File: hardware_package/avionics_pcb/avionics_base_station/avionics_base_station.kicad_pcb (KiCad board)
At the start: 2 copper layers, 33 x 52.7 mm, 9 parts, among them J1 ANT, J2 GND_PASS, U1 NODEMCU, U2 RFM98

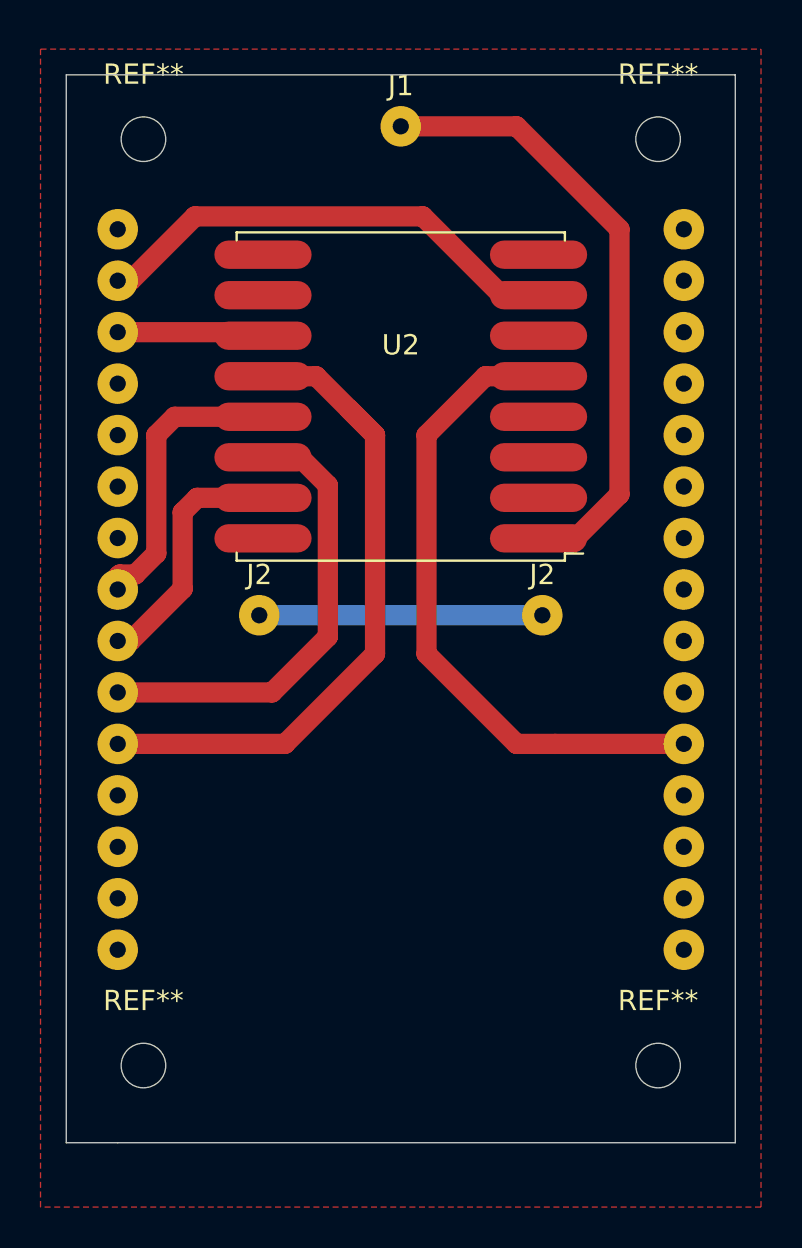
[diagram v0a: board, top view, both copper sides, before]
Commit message: updated the base station PCB
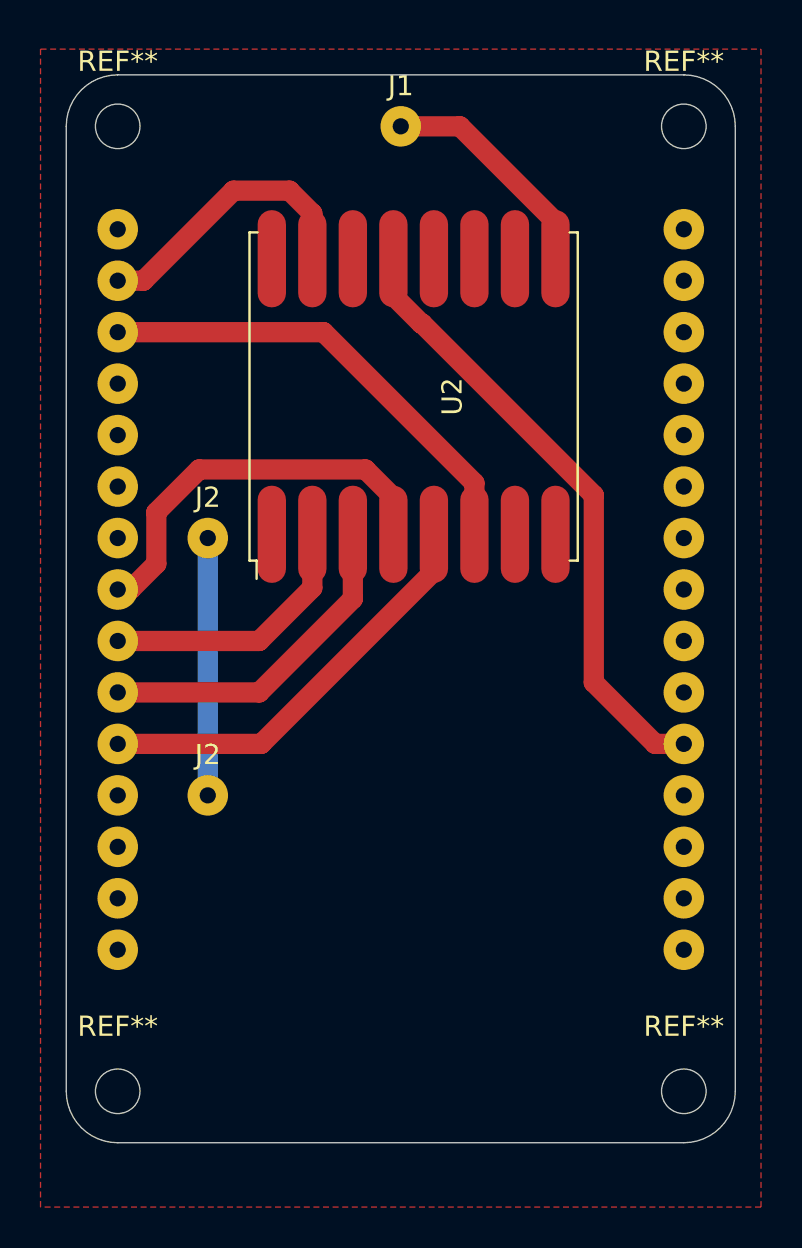
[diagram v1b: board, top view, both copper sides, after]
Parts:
- removed the REF** at (67.3, 38.7)
- removed the REF** at (41.9, 38.7)
- removed the REF** at (67.3, 84.5)
- added REF**: MountingHole_2.2mm_M2, MountingHole:MountingHole_2.2mm_M2, F.Cu at (68.6, 38.1)
- added REF**: MountingHole_2.2mm_M2, MountingHole:MountingHole_2.2mm_M2, F.Cu at (40.6, 38.1)
- added REF**: M2, MountingHole:MountingHole_2.2mm_M2, F.Cu at (68.6, 85.7)
- moved J2 18.8 mm to (45.1, 71.1)
- moved J2 4.58 mm to (45.1, 58.4)
- moved REF** 1.80 mm to (40.6, 85.7)
- moved U2 0.63 mm to (55.2, 51.4), turned to 90 degrees
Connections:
- U2 pad 1: Net-(J1-Pad1) -> GND
- U2 pad 10: (no net) -> GND
- U2 pad 11: Net-(U1-Pad13) -> (no net)
- U2 pad 12: Net-(U1-Pad5) -> (no net)
- U2 pad 13: Net-(U1-Pad8) -> +3V3
- U2 pad 14: Net-(U1-Pad6) -> (no net)
- U2 pad 15: Net-(U1-Pad7) -> Net-(U1-Pad14)
- U2 pad 16: GND -> (no net)
- U2 pad 2: GND -> Net-(U1-Pad7)
- U2 pad 3: (no net) -> Net-(U1-Pad6)
- U2 pad 4: (no net) -> Net-(U1-Pad8)
- U2 pad 5: +3V3 -> Net-(U1-Pad5)
- U2 pad 6: (no net) -> Net-(U1-Pad13)
- U2 pad 7: Net-(U1-Pad14) -> (no net)
- U2 pad 8: (no net) -> GND
- U2 pad 9: GND -> Net-(J1-Pad1)
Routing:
- net Net-(J1-Pad1): track 29.7 -> 10.2 mm
- net Net-(U1-Pad13): track 6.04 -> 24.4 mm
- net Net-(U1-Pad5): track 35.1 -> 19.8 mm
- net Net-(U1-Pad14): track 24.9 -> 12.9 mm
- net Net-(U1-Pad6): track 24.0 -> 15.5 mm
- net Net-(U1-Pad8): track 13.3 -> 21.1 mm
- net +3V3: track 33.3 -> 31.9 mm
- net GND: track 14.0 -> 12.7 mm
- net Net-(U1-Pad7): track 11.1 -> 12.1 mm
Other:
- outline, holes or cut-outs redrawn
